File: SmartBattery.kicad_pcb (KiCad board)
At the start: 4 copper layers, 100 x 80 mm, 413 parts, among them J1 USB_C_Receptacle_USB2.0, J10 JST 2P-1.0, J11 JST 2P-1.0, J12 Conn_01x10_Male, J13 Conn_01x03_Male, J15 USB_C_Receptacle_USB2.0, J2 ST-USB-003A, J3 JACK-C-PC-10A-RA(R), J4 JST 2P-1.0, J5 JST 2P-1.0, J6 JST 2P-1.0, J7 JST 2P-1.0, J8 JST 2P-1.0, J9 JST 2P-1.0, Q1 VBA2625, Q10 AON7400A, Q11 AON7400A, Q12 BSC067N06LS3, Q13 BSC067N06LS3, Q14 2n7002K, Q15 VBA2625, Q16 VBA2625, Q17 VBA2625, Q18 VBA2625, Q19 VBA2625, Q2 2n7002K, Q20 VBA2625, Q21 2n7002K, Q22 AO3401A, Q23 VBA2625, Q24 VBA2625, Q25 2n7002K, Q26 VBA2625, Q27 VBA2625, Q3 AON7400A, Q4 AON7400A, Q5 AON7400A, Q6 AON7400A, Q7 2n7002K, Q8 AON7400A, Q9 AON7400A, SW1 SW_Push, SW2 SW_Push, SW3 SW_Push, SW4 SW_Push, U1 BQ25703ARSNR, U10 ESP32-WROOM-32U, U11 STUSB4500, U12 STUSB4700, U13 TPS2511DGNR, U14 HT7533-1, U15 LMR14030SDDAR, U2 BQ294706DSGR, U3 ITV4030, U4 BQ40Z50, U5 LM5175PWPR, U6 STM32F730R8T6, U7 W25Q128JVSIQ, U8 LMR14030SDDAR, U9 FS35ND01G-S1Y2QWFI000, Y1 Q13FC1350000400, Y2 Crystal_GND24

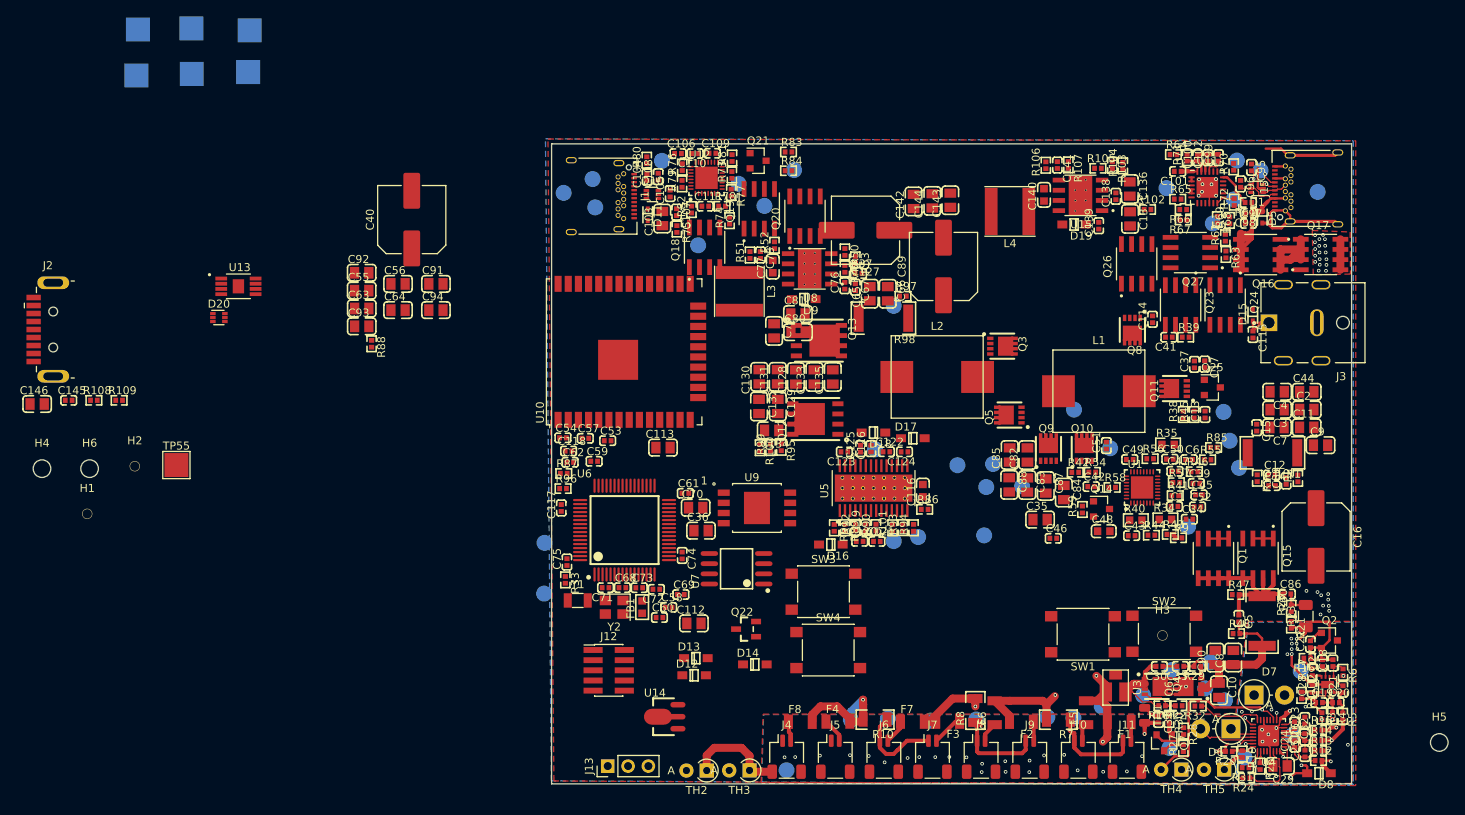
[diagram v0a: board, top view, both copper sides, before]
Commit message: Much layout wow.
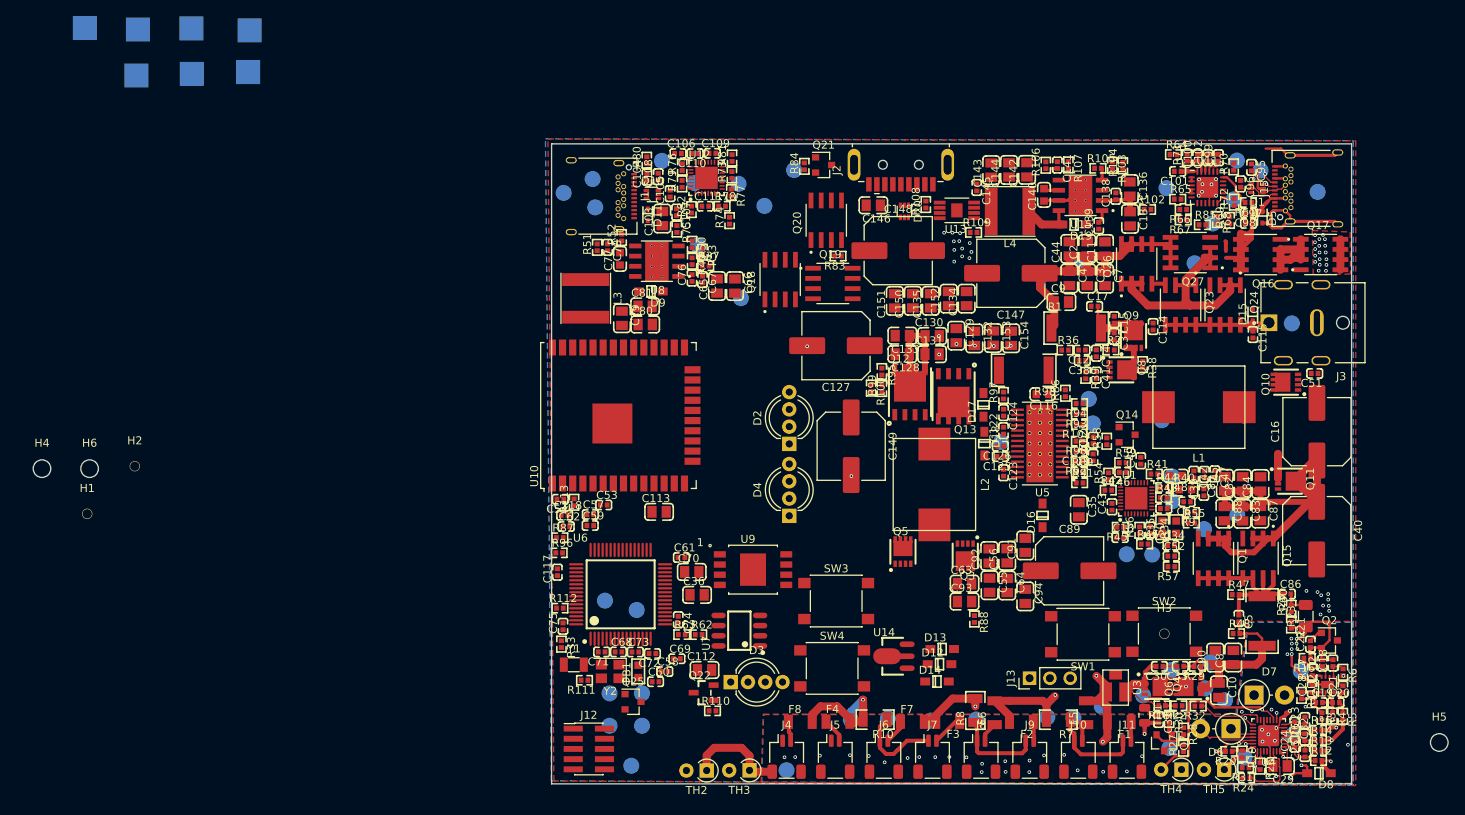
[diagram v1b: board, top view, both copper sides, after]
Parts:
- added C147: 220u, Capacitor_SMD:C_Elec_8x10.2, F.Cu at (57.4, 16.2)
- added C148: 220u, Capacitor_SMD:C_Elec_8x10.2, F.Cu at (43.3, 13.3)
- added C149: 220u, Capacitor_SMD:C_Elec_8x10.2, F.Cu at (37.5, 37.8)
- added C150: 22u, lc_lib:0805_C, F.Cu at (45.2, 19.6)
- added C151: 22u, lc_lib:0805_C, F.Cu at (42.9, 19.6)
- added C152: 22u, lc_lib:0805_C, F.Cu at (49.6, 19.4)
- added C153: 22u, lc_lib:0805_C, F.Cu at (55.2, 24.3)
- added C154: 22u, lc_lib:0805_C, F.Cu at (57.4, 24.3)
- added D2: LED_BARG, LED_THT:LED_D5.0mm-4_RGB_Wide_Pins, F.Cu at (29.7, 37.5)
- added D3: LED_BARG, LED_THT:LED_D5.0mm-4_RGB_Wide_Pins, F.Cu at (22.4, 67.3)
- added D4: LED_BARG, LED_THT:LED_D5.0mm-4_RGB_Wide_Pins, F.Cu at (29.7, 46.5)
- added R110: 100k, lc_lib:0402_R, F.Cu at (20.1, 70.9)
- added R111: 100k, lc_lib:0402_R, F.Cu at (4.12, 67.0)
- added R112: 100k, lc_lib:0402_R, F.Cu at (1.04, 58.0)
- added R113: 100k, lc_lib:0402_R, F.Cu at (2.81, 44.8)
- added TP56: TestPoint, TestPoint:TestPoint_Pad_D2.0mm, B.Cu at (7.25, 72.7)
- added TP57: TestPoint, TestPoint:TestPoint_Pad_D2.0mm, B.Cu at (11.3, 72.7)
- added TP58: TestPoint, TestPoint:TestPoint_Pad_D2.0mm, B.Cu at (7.25, 68.7)
- added TP59: TestPoint, TestPoint:TestPoint_Pad_D2.0mm, B.Cu at (11.3, 68.7)
- added TP60: TestPoint, TestPoint:TestPoint_Pad_D2.0mm, B.Cu at (9.96, 77.7)
- J12: value Conn_01x10_Male -> Conn_02x05_Odd_Even
- TP55: moved to B.Cu
- U7: value W25Q128JVSIQ -> LY68L6400SLIT; footprint lc_lib:SOP-8_208MIL -> lc_lib:SOP-8_150MIL
- moved C40 119.6 mm to (95.6, 48.4), turned to 270 degrees
- moved C145 116.6 mm to (53.1, 5.46), turned to 270 degrees
- moved R109 108.9 mm to (52.8, 11.1)
- moved J2 108.5 mm to (43.7, 3.29), turned to 90 degrees
- moved C146 107.4 mm to (40.2, 7.68), turned to 180 degrees
- moved R108 106.8 mm to (46.8, 7.58), turned to 90 degrees
- moved U13 90.3 mm to (50.7, 8.31), turned to 180 degrees
- moved D20 86.7 mm to (44.1, 8.44), turned to 270 degrees
- moved C55 86.7 mm to (54.8, 55.2), turned to 270 degrees
- moved C92 86.1 mm to (54.7, 51.5), turned to 90 degrees
- moved C64 83.6 mm to (57.0, 55.2), turned to 270 degrees
- moved C56 83.4 mm to (57.0, 51.5), turned to 90 degrees
- moved R63 83.0 mm to (16.3, 61.3), turned to 0 degrees
- moved C93 82.8 mm to (51.6, 57.2)
- moved R88 82.8 mm to (52.9, 59.4)
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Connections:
- net /MCU/QUADSPI_BK2_NCS renamed Net-(U6-Pad52)
- net /type_c_input/INPUT_TYPEC_VBUS_DIV7 renamed Net-(R62-Pad1)
- net Net-(U10-Pad25) renamed /MCU/ESP32_SERIAL_BL
- net Net-(U10-Pad26) renamed /MCU/ESP32_WAKE
- net Net-(U10-Pad33) renamed /MCU/ESP32_SDA
- net Net-(U10-Pad34) renamed /MCU/ESP32_UART_RX
- net Net-(U10-Pad35) renamed /MCU/ESP32_UART_TX
- net Net-(U10-Pad36) renamed /MCU/ESP32_SCL
- net Net-(U6-Pad10) renamed /MCU/ADC1_IN12
- net Net-(U6-Pad11) renamed /MCU/ADC1_IN13
- net Net-(U6-Pad20) renamed /MCU/DAC1
- net Net-(U6-Pad21) renamed /MCU/DAC2
- net Net-(U6-Pad24) renamed /MCU/ADC1_IN14
- net Net-(U6-Pad28) renamed /MCU/I2C2_SCL
- net Net-(U6-Pad29) renamed /MCU/I2C2_SDA
- net Net-(U6-Pad44) renamed /MCU/USB_FS_DM
- net Net-(U6-Pad45) renamed /MCU/USB_FS_DP
- net Net-(U6-Pad53) renamed /MCU/UART5_TX
- net Net-(U6-Pad54) renamed /MCU/UART5_RX
- net Net-(U6-Pad57) renamed /MCU/I2C1_SMBA
- net Net-(U6-Pad59) renamed /MCU/I2C1_SDA
- net Net-(U6-Pad61) renamed /MCU/I2C1_SCL
- net Net-(U6-Pad8) renamed /MCU/ADC1_IN10
- net Net-(U6-Pad9) renamed /MCU/ADC1_IN11
- C101 pad 1: Net-(C101-Pad1) -> /type_c_input/INPUT_TYPEC_VBUS_RAW
- C112 pad 1: Net-(C112-Pad1) -> GND
- C113 pad 1: Net-(C113-Pad1) -> GND
- C127 pad 1: GND -> /Type_C_Output/OUTPUT_TYPEC_PWR
- C127 pad 2: /Type_C_Output/OUTPUT_TYPEC_PWR -> GND
- C36 pad 2: /Peripheral_3p3v/3p3v -> +3.3VP
- C40 pad 1: GND -> /Charger/VSYS
- C40 pad 2: /Charger/VSYS -> GND
- C53 pad 1: /Peripheral_3p3v/3p3v -> +3.3VP
- C54 pad 1: /Peripheral_3p3v/3p3v -> +3.3VP
- C57 pad 1: /Peripheral_3p3v/3p3v -> +3.3VP
- C59 pad 1: /Peripheral_3p3v/3p3v -> +3.3VP
- C61 pad 1: /Peripheral_3p3v/3p3v -> +3.3VP
- C62 pad 1: /Peripheral_3p3v/3p3v -> +3.3VP
- C74 pad 1: /Peripheral_3p3v/3p3v -> +3.3VP
- C75 pad 1: /Peripheral_3p3v/3p3v -> +3.3VP
- C97 pad 2: Net-(C101-Pad1) -> /type_c_input/INPUT_TYPEC_VBUS_RAW
- C98 pad 1: Net-(C101-Pad1) -> /type_c_input/INPUT_TYPEC_VBUS_RAW
- D12 pad 1: Net-(D12-Pad1) -> Net-(C112-Pad2)
- D12 pad 2: Net-(D12-Pad2) -> /Barrel_Jack_Input/BARREL_RAW
- D13 pad 1: Net-(D13-Pad1) -> +3.3VP
- D13 pad 2: Net-(D13-Pad2) -> Net-(C113-Pad2)
- D14 pad 1: Net-(D14-Pad1) -> Net-(C112-Pad2)
- D14 pad 2: Net-(D14-Pad2) -> /type_c_input/INPUT_TYPEC_VBUS_RAW
- D5 pad 2: Net-(C101-Pad1) -> /type_c_input/INPUT_TYPEC_VBUS_RAW
- FB1 pad 1: /Peripheral_3p3v/3p3v -> +3.3VP
- J12 pad 1: Net-(J12-Pad1) -> +3.3VP
- J12 pad 10: Net-(J12-Pad10) -> /MCU/NRST
- J12 pad 2: Net-(J12-Pad2) -> /MCU/SWDIO
- J12 pad 3: Net-(J12-Pad3) -> GND
- J12 pad 4: Net-(J12-Pad4) -> /MCU/SWDCLK
- J12 pad 5: Net-(J12-Pad5) -> GND
- J12 pad 6: Net-(J12-Pad6) -> /MCU/SWO
- J15 pad A4: Net-(C101-Pad1) -> /type_c_input/INPUT_TYPEC_VBUS_RAW
- J15 pad A9: Net-(C101-Pad1) -> /type_c_input/INPUT_TYPEC_VBUS_RAW
- J15 pad B4: Net-(C101-Pad1) -> /type_c_input/INPUT_TYPEC_VBUS_RAW
- J15 pad B9: Net-(C101-Pad1) -> /type_c_input/INPUT_TYPEC_VBUS_RAW
- Q10 pad 1: Net-(Q10-Pad1) -> GND
- Q10 pad 2: Net-(Q10-Pad1) -> GND
- Q10 pad 3: Net-(Q10-Pad1) -> GND
- Q10 pad 4: Net-(Q10-Pad4) -> Net-(C51-Pad2)
- Q12 pad 0: (no net) -> /Type_C_Output/OUTPUT_TYPEC_PWR
- Q13 pad 0: (no net) -> /OutputStage/SW2
- Q16 pad 5: Net-(C101-Pad1) -> /type_c_input/INPUT_TYPEC_VBUS_RAW
- Q16 pad 6: Net-(C101-Pad1) -> /type_c_input/INPUT_TYPEC_VBUS_RAW
- Q16 pad 7: Net-(C101-Pad1) -> /type_c_input/INPUT_TYPEC_VBUS_RAW
- Q16 pad 8: Net-(C101-Pad1) -> /type_c_input/INPUT_TYPEC_VBUS_RAW
- Q22 pad 2: Net-(Q22-Pad2) -> +3.3VP
- Q22 pad 3: Net-(Q22-Pad3) -> /Peripheral_3p3v/3p3v
- R33 pad 1: /Peripheral_3p3v/3p3v -> +3.3VP
- R61 pad 1: Net-(C101-Pad1) -> /type_c_input/INPUT_TYPEC_VBUS_RAW
- R63 pad 2: Net-(C101-Pad1) -> Net-(R63-Pad2)
- SW3 pad 1: Net-(SW3-Pad1) -> /MCU/NRST
- SW3 pad 2: Net-(SW3-Pad2) -> GND
- SW4 pad 1: Net-(SW4-Pad1) -> /MCU/BOOT
- SW4 pad 2: Net-(SW4-Pad2) -> +3.3VP
- TP31 pad 1: Net-(C101-Pad1) -> /type_c_input/INPUT_TYPEC_VBUS_RAW
- U10 pad 2: Net-(U10-Pad2) -> +3.3VP
- U10 pad 3: Net-(U10-Pad3) -> /MCU/GPIO_ENABLE_ESP32
- U11 pad 24: Net-(C101-Pad1) -> /type_c_input/INPUT_TYPEC_VBUS_RAW
- U14 pad 1: Net-(U14-Pad1) -> GND
- U14 pad 2: Net-(U14-Pad2) -> Net-(C112-Pad2)
- U14 pad 3: Net-(U14-Pad3) -> Net-(C113-Pad2)
- U6 pad 19: /Peripheral_3p3v/3p3v -> +3.3VP
- U6 pad 32: /Peripheral_3p3v/3p3v -> +3.3VP
- U6 pad 34: Net-(U6-Pad34) -> /MCU/SPI2_SCK
- U6 pad 35: Net-(U6-Pad35) -> /MCU/SPI2_MISO
- U6 pad 36: Net-(U6-Pad36) -> /MCU/SPI2_MOSI
- U6 pad 46: Net-(U6-Pad46) -> /MCU/SWDIO
- U6 pad 48: /Peripheral_3p3v/3p3v -> +3.3VP
- U6 pad 49: Net-(U6-Pad49) -> /MCU/SWDCLK
- U6 pad 55: Net-(U6-Pad55) -> /MCU/SWO
- U6 pad 60: Net-(U6-Pad60) -> /MCU/BOOT
- U6 pad 64: /Peripheral_3p3v/3p3v -> +3.3VP
- U6 pad 7: Net-(U6-Pad7) -> /MCU/NRST
- U7 pad 1: Net-(U7-Pad1) -> /MCU/QUASPI_BK1_NCS
- U7 pad 2: Net-(U7-Pad2) -> /MCU/QUADSPI_BK1_IO1
- U7 pad 5: Net-(U7-Pad5) -> /MCU/QUADSPI_BK1_IO0
- U7 pad 6: Net-(U7-Pad6) -> /MCU/QUADSPI_CLK
- U7 pad 8: /Peripheral_3p3v/3p3v -> +3.3VP
- U9 pad 2: Net-(U9-Pad2) -> /MCU/SPI2_MOSI
- U9 pad 5: Net-(U9-Pad5) -> /MCU/SPI2_MISO
- U9 pad 6: Net-(U9-Pad6) -> /MCU/SPI2_SCK
- U9 pad 8: /Peripheral_3p3v/3p3v -> +3.3VP
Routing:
- net /Charger/VSYS: track 5.08 -> 56.9 mm
- net /Charger/ADAPTER_IN: track 3.81 -> 43.4 mm
- net Net-(Q23-Pad1): track 0.00 -> 33.3 mm
- net /type_c_input/INPUT_TYPEC_VBUS_RAW: track 0.00 -> 32.9 mm
- net Net-(C101-Pad1): track 30.9 -> 0.00 mm
- net /Type_C_Output/OUTPUT_TYPEC_PWR: track 0.00 -> 26.0 mm
- net /Barrel_Jack_Input/BARREL_RAW: track 5.82 -> 19.5 mm
- net Net-(C15-Pad2): track 0.00 -> 10.7 mm
- net /Peripheral_3p3v/5v0_SWITCHED_NODE: track 0.00 -> 6.78 mm
- net Net-(C43-Pad1): track 0.00 -> 5.89 mm
- net /Peripheral_3p3v/VSYS_IN_5p0: track 0.00 -> 5.65 mm
- net GND: track 45.7 -> 50.6 mm, vias 16 -> 36
- net Net-(C46-Pad1): track 0.00 -> 4.09 mm
- net Net-(C140-Pad2): track 0.00 -> 1.94 mm
- net Net-(Q23-Pad4): track 0.00 -> 1.76 mm
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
